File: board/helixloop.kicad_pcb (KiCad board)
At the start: 2 copper layers, 128 x 128 mm, 308 parts

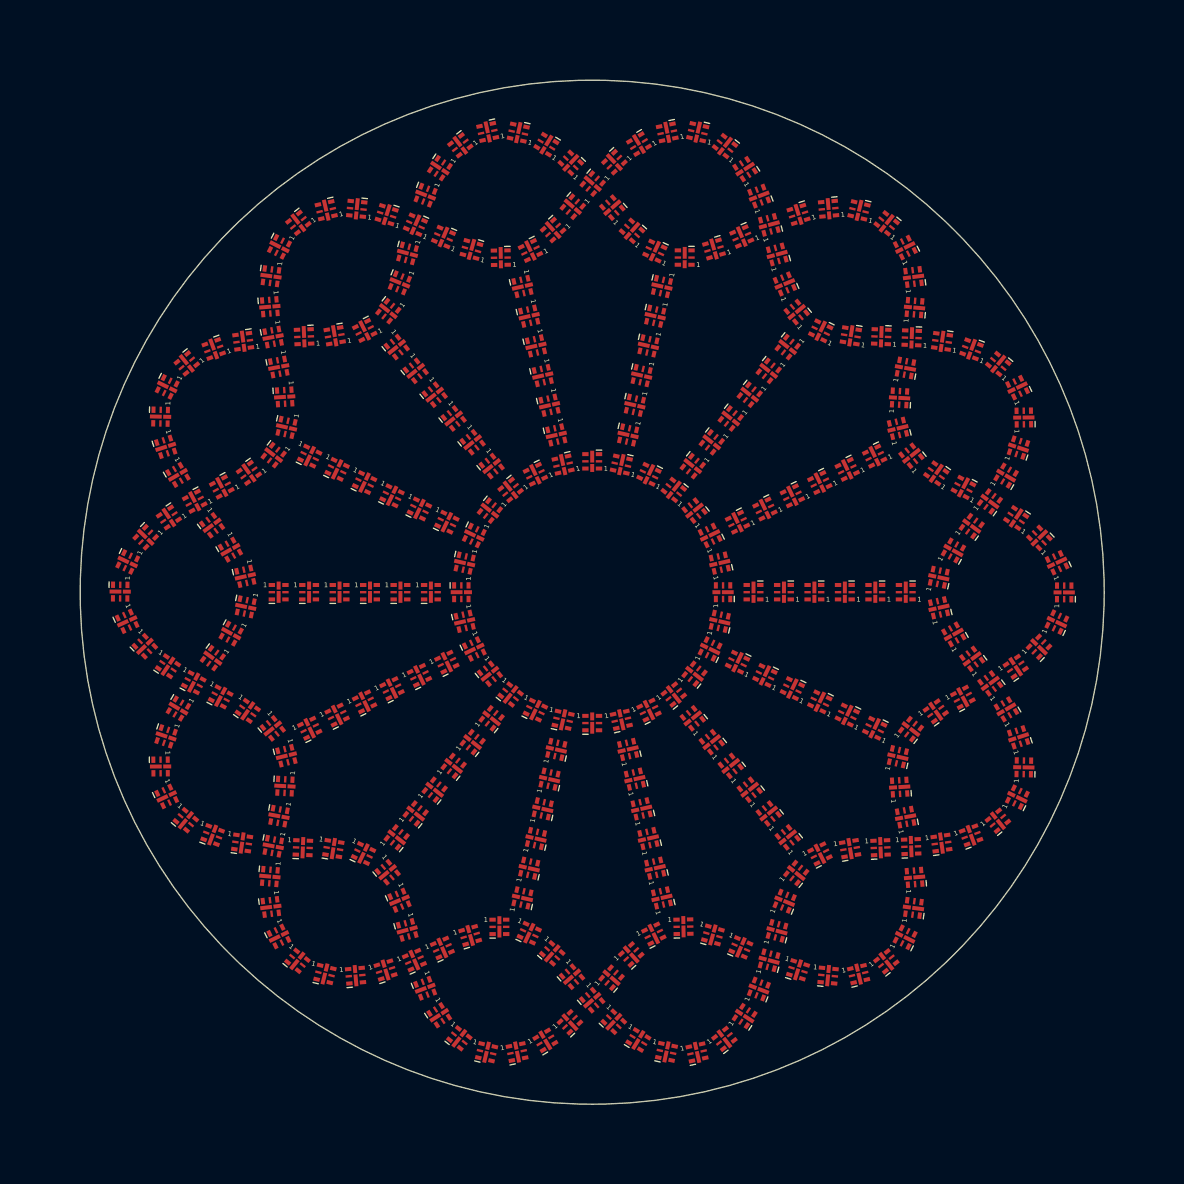
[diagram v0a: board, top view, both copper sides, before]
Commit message: a rather awesome revision
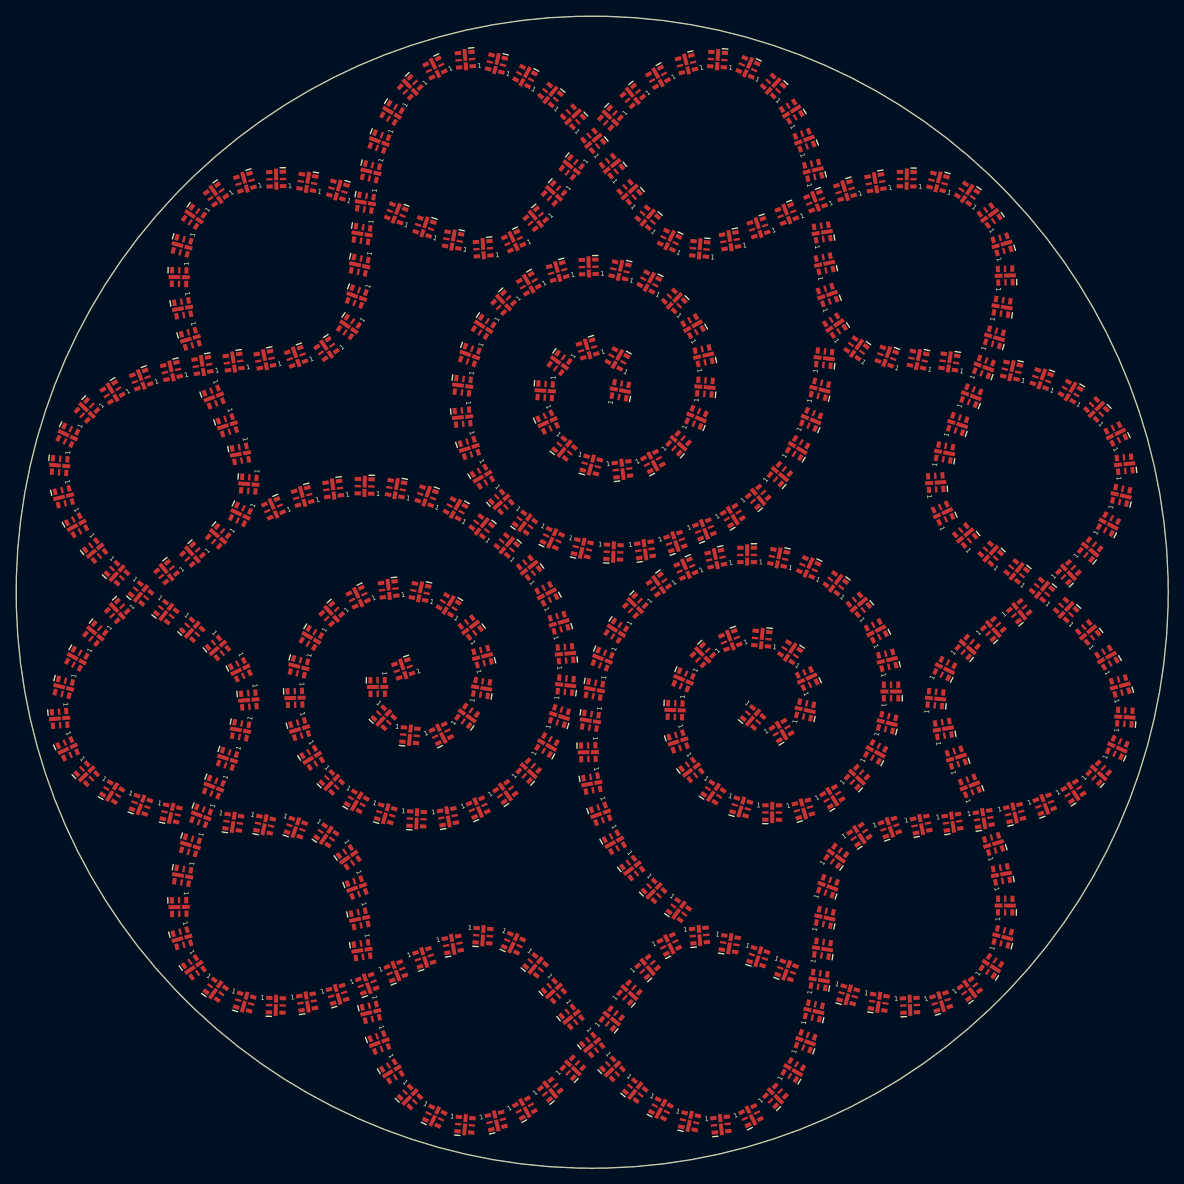
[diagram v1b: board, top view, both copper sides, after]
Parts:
- removed D121, D132, D141, D152, D161, D172, D181, D201, D212, D221, D232: LED-APA102-2020, LED-APA102-2020
- added D162: LED-APA102-2020, LED-APA102-2020, F.Cu at (127.6, 47.3)
- added D170: LED-APA102-2020, LED-APA102-2020, F.Cu at (105.1, 38.0)
- added D177: LED-APA102-2020, LED-APA102-2020, F.Cu at (86.4, 57.1)
- added D185: LED-APA102-2020, LED-APA102-2020, F.Cu at (56.6, 48.8)
- added D200: LED-APA102-2020, LED-APA102-2020, F.Cu at (46.8, 97.5)
- added D207: LED-APA102-2020, LED-APA102-2020, F.Cu at (34.4, 119.6)
- added D215: LED-APA102-2020, LED-APA102-2020, F.Cu at (63.0, 129.4)
- added D222: LED-APA102-2020, LED-APA102-2020, F.Cu at (72.3, 152.5)
- added D230: LED-APA102-2020, LED-APA102-2020, F.Cu at (94.8, 162.2)
- added D237: LED-APA102-2020, LED-APA102-2020, F.Cu at (113.4, 142.9)
- added D245: LED-APA102-2020, LED-APA102-2020, F.Cu at (124.7, 107.5)
- added D252: LED-APA102-2020, LED-APA102-2020, F.Cu at (112.4, 122.2)
- added D260: LED-APA102-2020, LED-APA102-2020, F.Cu at (136.9, 116.3)
- added D323: LED-APA102-2020, LED-APA102-2020, F.Cu at (71.5, 86.8)
- added D324: LED-APA102-2020, LED-APA102-2020, F.Cu at (67.6, 87.1)
- added D325: LED-APA102-2020, LED-APA102-2020, F.Cu at (63.8, 88.0)
- added D326: LED-APA102-2020, LED-APA102-2020, F.Cu at (60.2, 89.5)
- added D327: LED-APA102-2020, LED-APA102-2020, F.Cu at (103.5, 74.8)
- added D328: LED-APA102-2020, LED-APA102-2020, F.Cu at (103.1, 70.8)
- added D329: LED-APA102-2020, LED-APA102-2020, F.Cu at (99.4, 69.6)
- added D330: LED-APA102-2020, LED-APA102-2020, F.Cu at (95.9, 71.3)
- added D331: LED-APA102-2020, LED-APA102-2020, F.Cu at (94.1, 74.8)
- added D332: LED-APA102-2020, LED-APA102-2020, F.Cu at (94.4, 78.7)
- added D333: LED-APA102-2020, LED-APA102-2020, F.Cu at (96.5, 82.0)
- added D334: LED-APA102-2020, LED-APA102-2020, F.Cu at (99.9, 84.1)
- added D335: LED-APA102-2020, LED-APA102-2020, F.Cu at (103.8, 84.6)
- added D336: LED-APA102-2020, LED-APA102-2020, F.Cu at (107.6, 83.7)
- added D337: LED-APA102-2020, LED-APA102-2020, F.Cu at (110.8, 81.4)
- added D338: LED-APA102-2020, LED-APA102-2020, F.Cu at (113.0, 78.1)
- added D339: LED-APA102-2020, LED-APA102-2020, F.Cu at (114.1, 74.4)
- added D340: LED-APA102-2020, LED-APA102-2020, F.Cu at (113.9, 70.4)
- added D341: LED-APA102-2020, LED-APA102-2020, F.Cu at (112.6, 66.7)
- added D342: LED-APA102-2020, LED-APA102-2020, F.Cu at (110.3, 63.6)
- added D343: LED-APA102-2020, LED-APA102-2020, F.Cu at (107.1, 61.2)
- added D344: LED-APA102-2020, LED-APA102-2020, F.Cu at (103.5, 59.8)
- added D345: LED-APA102-2020, LED-APA102-2020, F.Cu at (99.6, 59.3)
- added D346: LED-APA102-2020, LED-APA102-2020, F.Cu at (95.7, 59.9)
- added D347: LED-APA102-2020, LED-APA102-2020, F.Cu at (92.1, 61.4)
- added D348: LED-APA102-2020, LED-APA102-2020, F.Cu at (88.9, 63.8)
- added D349: LED-APA102-2020, LED-APA102-2020, F.Cu at (86.4, 66.8)
- added D350: LED-APA102-2020, LED-APA102-2020, F.Cu at (84.7, 70.4)
- added D351: LED-APA102-2020, LED-APA102-2020, F.Cu at (83.8, 74.2)
- added D352: LED-APA102-2020, LED-APA102-2020, F.Cu at (83.8, 78.1)
- added D353: LED-APA102-2020, LED-APA102-2020, F.Cu at (84.6, 82.0)
- added D354: LED-APA102-2020, LED-APA102-2020, F.Cu at (86.3, 85.6)
- added D355: LED-APA102-2020, LED-APA102-2020, F.Cu at (88.6, 88.7)
- added D356: LED-APA102-2020, LED-APA102-2020, F.Cu at (91.6, 91.3)
- added D357: LED-APA102-2020, LED-APA102-2020, F.Cu at (95.0, 93.3)
- added D358: LED-APA102-2020, LED-APA102-2020, F.Cu at (98.8, 94.5)
- added D359: LED-APA102-2020, LED-APA102-2020, F.Cu at (102.7, 95.0)
- added D360: LED-APA102-2020, LED-APA102-2020, F.Cu at (106.6, 94.7)
- added D361: LED-APA102-2020, LED-APA102-2020, F.Cu at (110.4, 93.7)
- added D362: LED-APA102-2020, LED-APA102-2020, F.Cu at (114.0, 92.2)
- added D363: LED-APA102-2020, LED-APA102-2020, F.Cu at (117.6, 90.4)
- added D364: LED-APA102-2020, LED-APA102-2020, F.Cu at (120.7, 88.1)
- added D365: LED-APA102-2020, LED-APA102-2020, F.Cu at (123.5, 85.2)
- added D366: LED-APA102-2020, LED-APA102-2020, F.Cu at (125.7, 82.0)
- added D367: LED-APA102-2020, LED-APA102-2020, F.Cu at (127.4, 78.4)
- added D368: LED-APA102-2020, LED-APA102-2020, F.Cu at (128.5, 74.6)
- added D369: LED-APA102-2020, LED-APA102-2020, F.Cu at (129.0, 70.7)
- moved D166 113.1 mm to (119.5, 34.4), turned to 155.398 degrees
- moved D167 112.2 mm to (115.7, 33.4), turned to 175.941 degrees
- moved D165 111.5 mm to (122.6, 36.7), turned to 136.612 degrees
- moved D168 109.2 mm to (111.8, 34.0), turned to -165.497 degrees
- moved D164 108.1 mm to (124.9, 39.9), turned to 121.691 degrees
- moved D146 107.1 mm to (166.6, 84.0), turned to 95.7431 degrees
- moved D169 105.0 mm to (108.2, 35.6), turned to -150.848 degrees
- moved D163 103.7 mm to (126.5, 43.5), turned to 110.771 degrees
- moved D147 103.5 mm to (165.5, 80.2), turned to 116.285 degrees
- moved D184 101.7 mm to (60.5, 48.4), turned to -178.549 degrees
- moved D183 101.7 mm to (64.4, 48.8), turned to 170.606 degrees
- moved D182 101.2 mm to (68.2, 49.7), turned to 163.354 degrees
- moved D186 100.3 mm to (53.0, 50.3), turned to -145.002 degrees
- moved D148 98.5 mm to (163.0, 77.2), turned to 134.789 degrees
- moved D187 98.2 mm to (50.2, 53.1), turned to -124.458 degrees
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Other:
- board size 128 x 128 mm -> 144 x 144 mm

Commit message: tweaks; make layout script
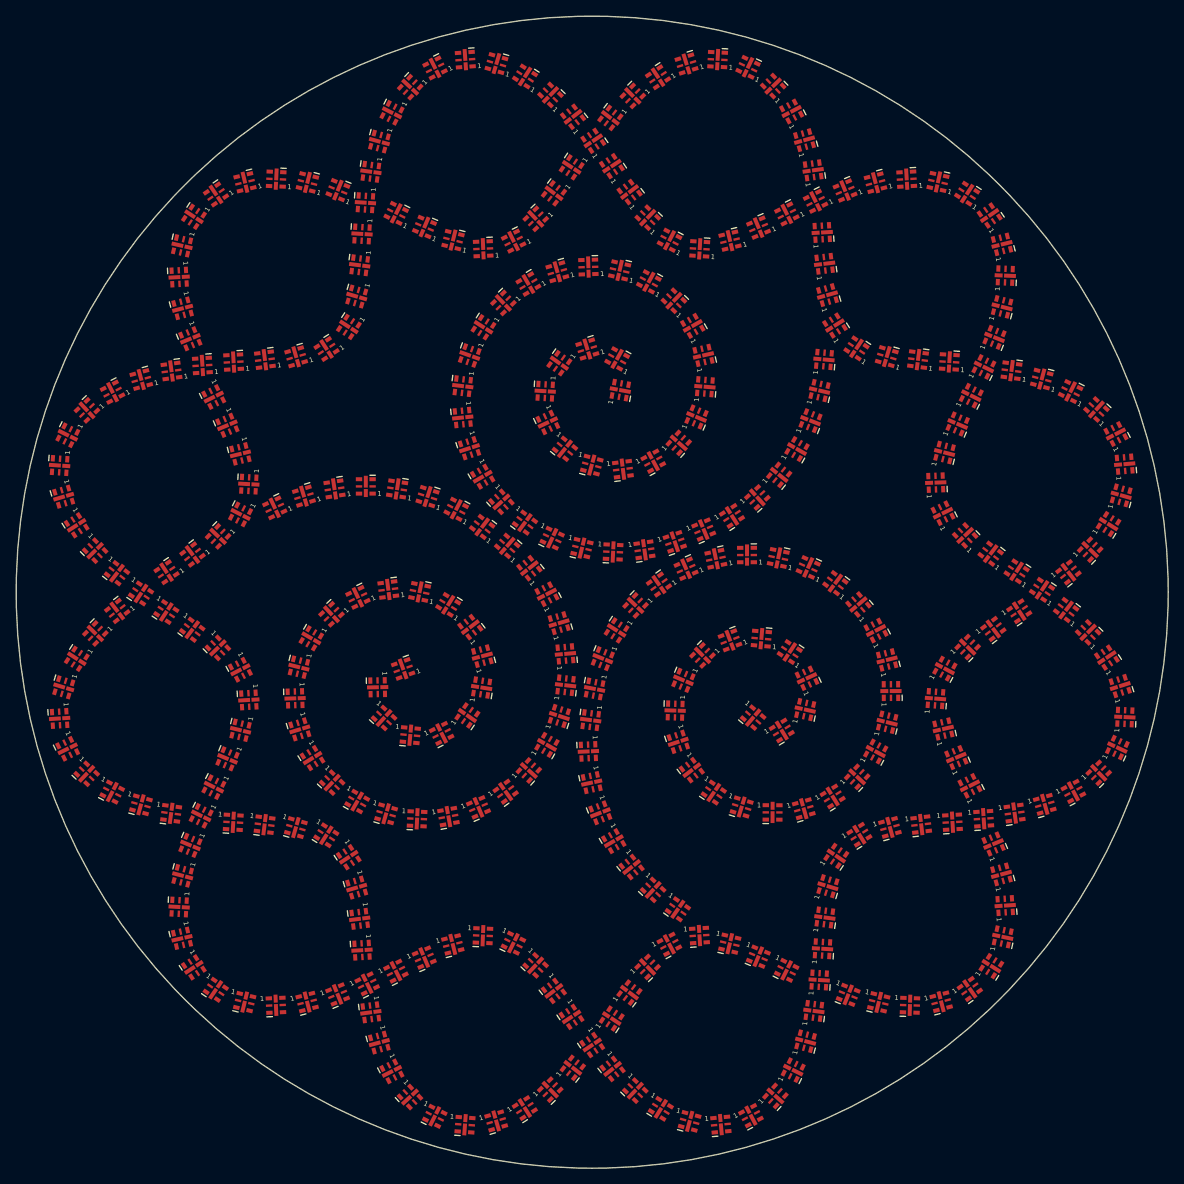
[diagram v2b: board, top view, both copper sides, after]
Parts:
- moved D283 0.17 mm to (110.7, 139.6), turned to -34.9995 degrees
- moved D326 0.17 mm to (60.3, 89.5), turned to -155 degrees
- moved D369 0.17 mm to (129.0, 70.9), turned to 85.0005 degrees
- moved D281 0.17 mm to (104.9, 134.4), turned to -51.395 degrees
- moved D367 0.17 mm to (127.3, 78.6), turned to 68.605 degrees
- moved D324 0.17 mm to (67.8, 87.1), turned to -171.395 degrees
- moved D368 0.16 mm to (128.4, 74.8), turned to 76.9221 degrees
- moved D325 0.16 mm to (64.0, 88.0), turned to -163.078 degrees
- moved D282 0.16 mm to (107.6, 137.2), turned to -43.0779 degrees
- moved D366 0.15 mm to (125.6, 82.1), turned to 60.0309 degrees
- moved D280 0.15 mm to (102.7, 131.1), turned to -59.9691 degrees
- moved D323 0.15 mm to (71.7, 86.8), turned to -179.969 degrees
- moved D279 0.13 mm to (101.0, 127.6), turned to -68.8186 degrees
- moved D322 0.13 mm to (75.6, 87.1), turned to 171.181 degrees
- moved D365 0.13 mm to (123.4, 85.3), turned to 51.1814 degrees
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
